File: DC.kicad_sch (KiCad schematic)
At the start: 5 parts, among them U1 LT8610, U2 LT3483AxS6, U3 LT3094xMSE, U4 ADP7118ACPZN, U5 ADP7118ACPZN

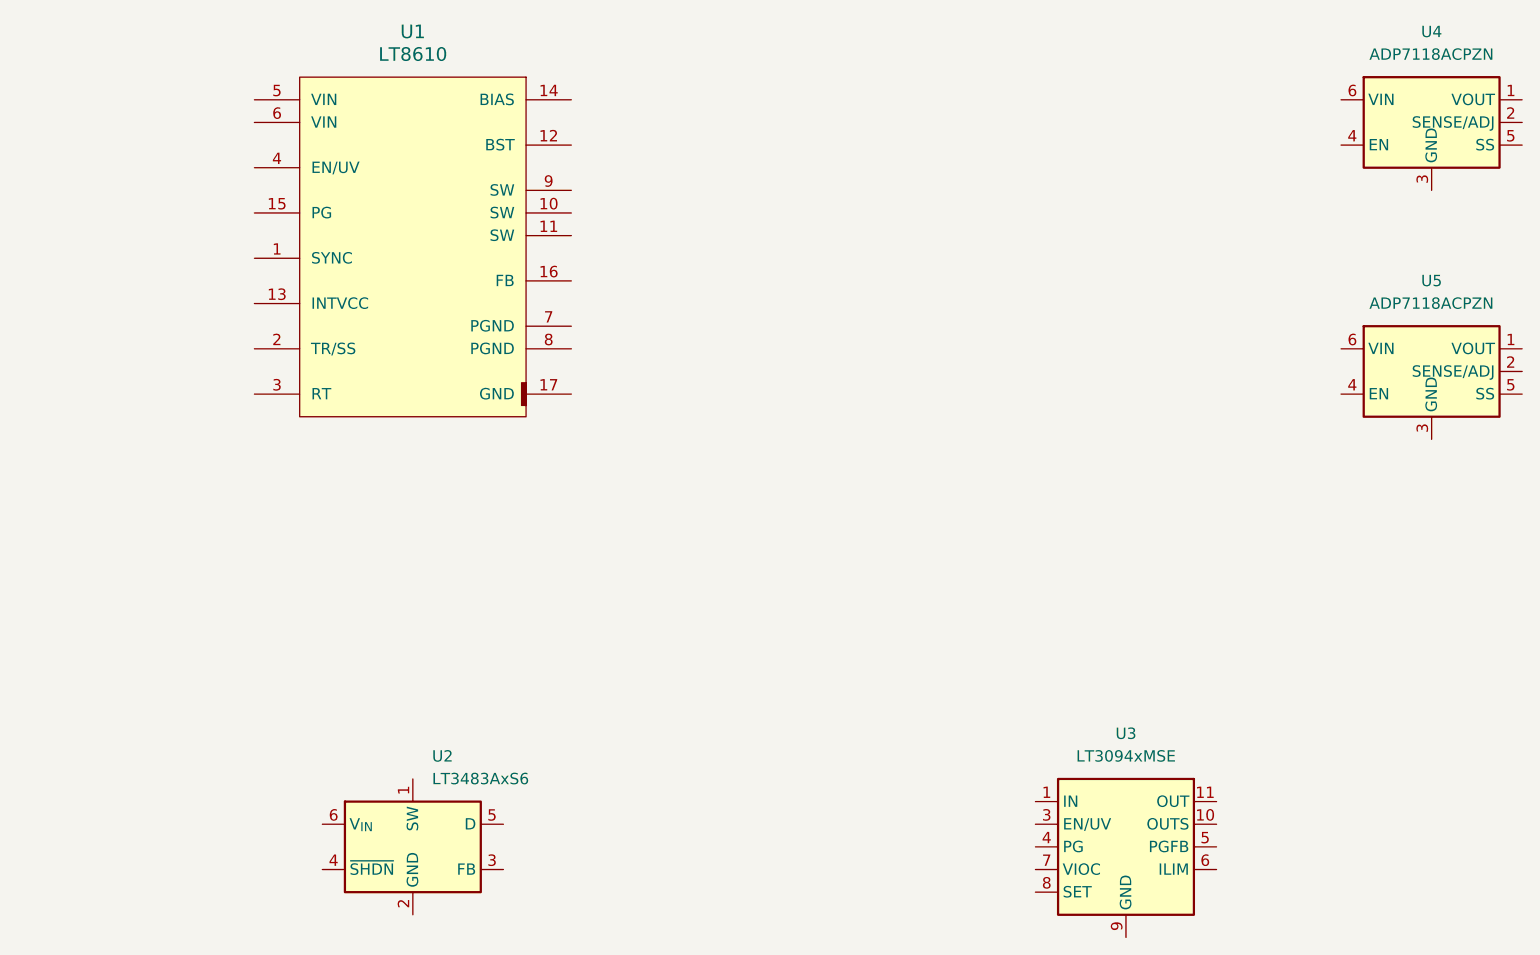
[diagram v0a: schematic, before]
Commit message: DC almost done
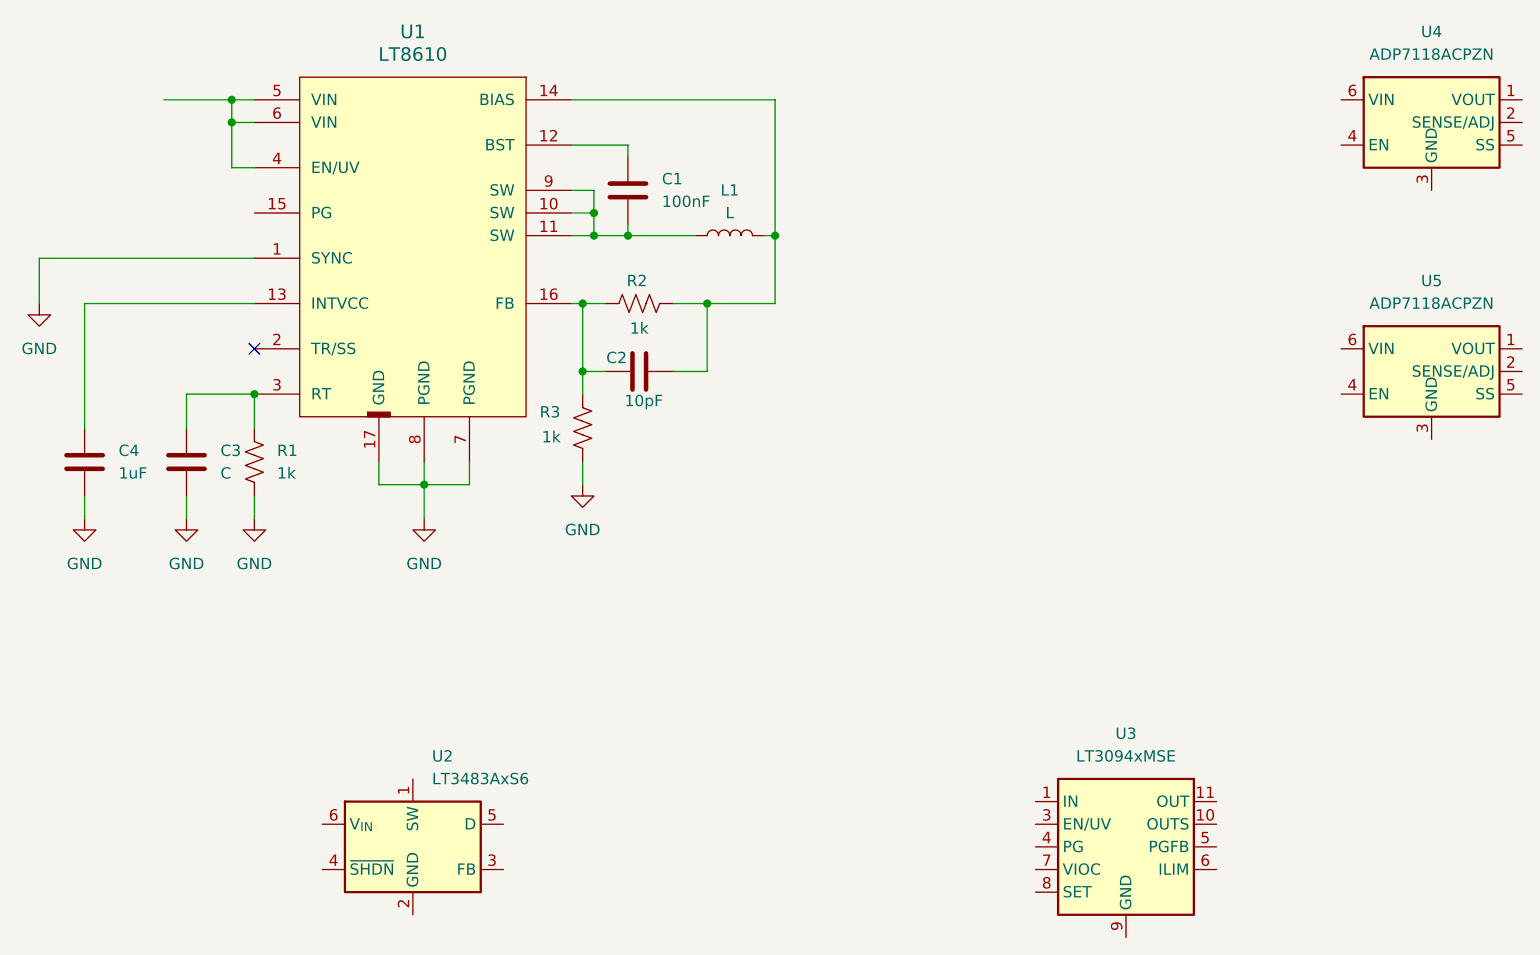
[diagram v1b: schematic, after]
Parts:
- added C1: 100nF, SparkFun-Resistor:R_0603_1608Metric, symbol Device:C
- added C2: 10pF, SparkFun-Resistor:R_0603_1608Metric, symbol Device:C
- added C3: C, symbol Device:C
- added C4: 1uF, symbol Device:C
- added L1: L, symbol Device:L
- added R1, R2, R3: 1k, SparkFun-Resistor:R_0603_1608Metric, symbol SparkFun:R
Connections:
- net GND: now reaches U1.1 (SYNC)
- net GND: now also U1.17 (GND), U1.7 (PGND), U1.8 (PGND), C3.2, C4.2, R1.2, R3.2
- net at U1.10 (SW): now also U1.11 (SW), U1.9 (SW), C1.2, L1.1
- net at U1.12 (BST): now also C1.1
- net at U1.13 (INTVCC): now also C4.1
- net at U1.14 (BIAS): now also C2.2, L1.2, R2.1
- net at U1.16 (FB): now also C2.1, R2.2, R3.1
- net at U1.3 (RT): now also C3.1, R1.1
- net at U1.4 (EN/UV): now also U1.5 (VIN), U1.6 (VIN)
- no-connect marks 0 -> 1
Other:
- moved on the sheet: U1
